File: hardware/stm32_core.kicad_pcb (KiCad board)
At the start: 2 copper layers, 36 parts, among them J8 I2C_HEADER,2.54, SW19 SW_RESET,2_leg,SMD, U10 STM32F103C8T6, Y2 O8M, Y3 O32.768K

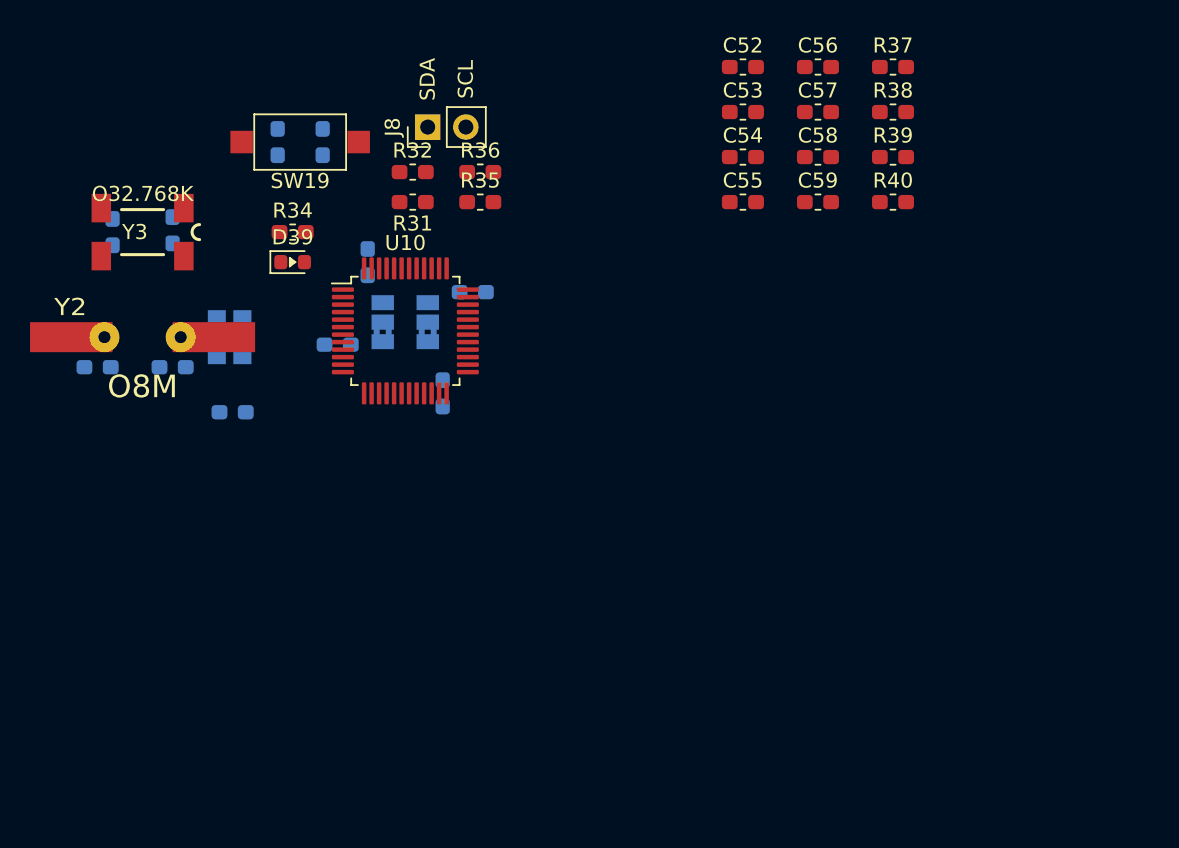
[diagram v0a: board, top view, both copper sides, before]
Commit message: update ws2812,
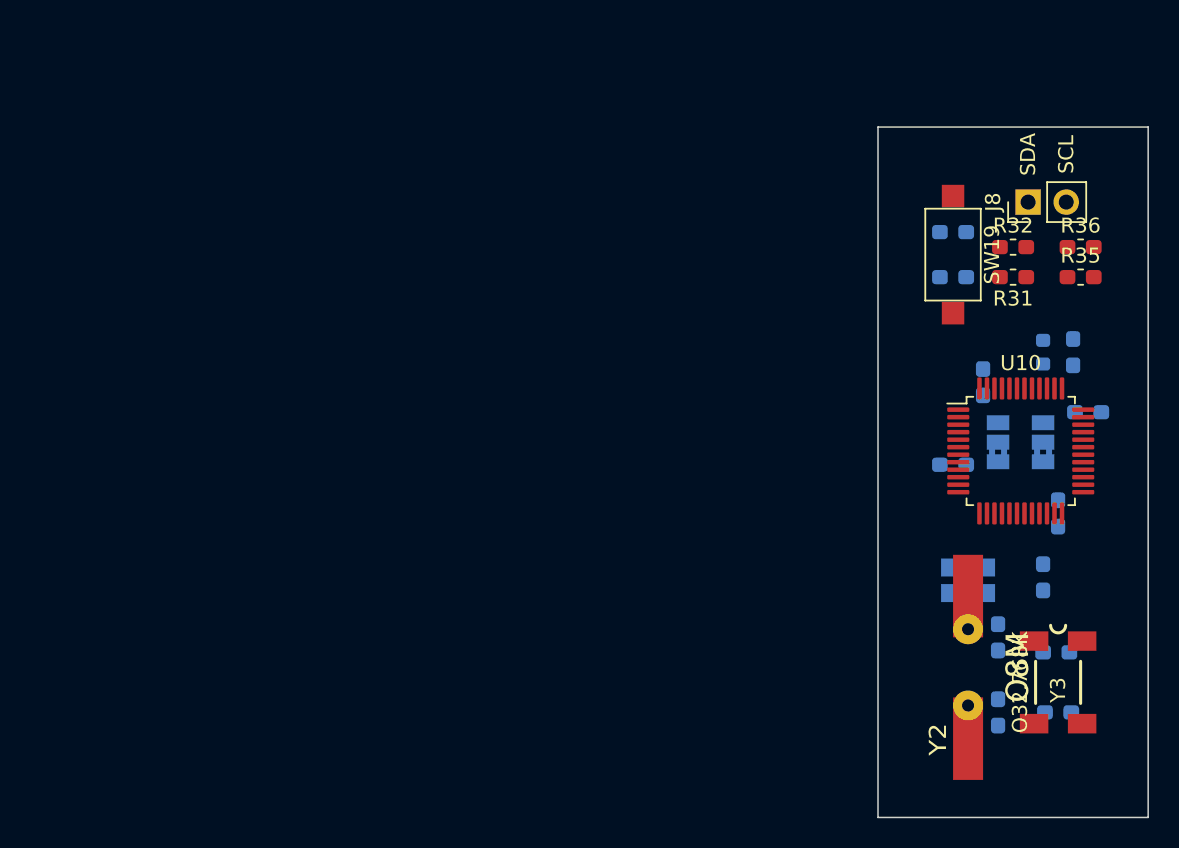
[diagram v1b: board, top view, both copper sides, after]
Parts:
- removed C52, C53, C54, C55, C56, C57, C58, C59: SPARE,0603, Capacitor_SMD:C_0603_1608Metric_Pad1.05x0.95mm_HandSolder
- removed R37, R38, R39, R40: R0,0603, Resistor_SMD:R_0603_1608Metric_Pad1.05x0.95mm_HandSolder
- D39, R34: moved to B.Cu
- moved C50 70.7 mm to (69.0, 56.0), turned to 0 degrees
- moved Y3 68.0 mm to (69.0, 54.0), turned to 270 degrees
- moved C49 65.2 mm to (68.9, 52.0), turned to 0 degrees
- moved C47 64.3 mm to (65.0, 56.0), turned to 90 degrees
- moved Y2 59.2 mm to (63.0, 53.0), turned to 90 degrees
- moved C48 57.9 mm to (65.0, 51.0), turned to 270 degrees
- moved C42 55.1 mm to (68.0, 47.0), turned to 270 degrees
- moved R34 52.6 mm to (70.0, 32.0), turned to 90 degrees
- moved D39 50.4 mm to (68.0, 32.0), turned to 90 degrees
- moved C43 45.9 mm to (62.0, 27.0), turned to 180 degrees
- moved SW19 44.1 mm to (62.0, 25.5), turned to 270 degrees
- moved R33 42.4 mm to (62.0, 24.0), turned to 180 degrees
- moved C44 41.8 mm to (62.0, 39.5)
- moved C45 41.8 mm to (64.0, 34.0)
- moved C46 41.8 mm to (71.0, 36.0)
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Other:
- board outline added: 18 x 46 mm
